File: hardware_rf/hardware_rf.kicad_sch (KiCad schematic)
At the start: 5 parts, among them IC1 CC1125RHBR, Y1 Crystal_GND24

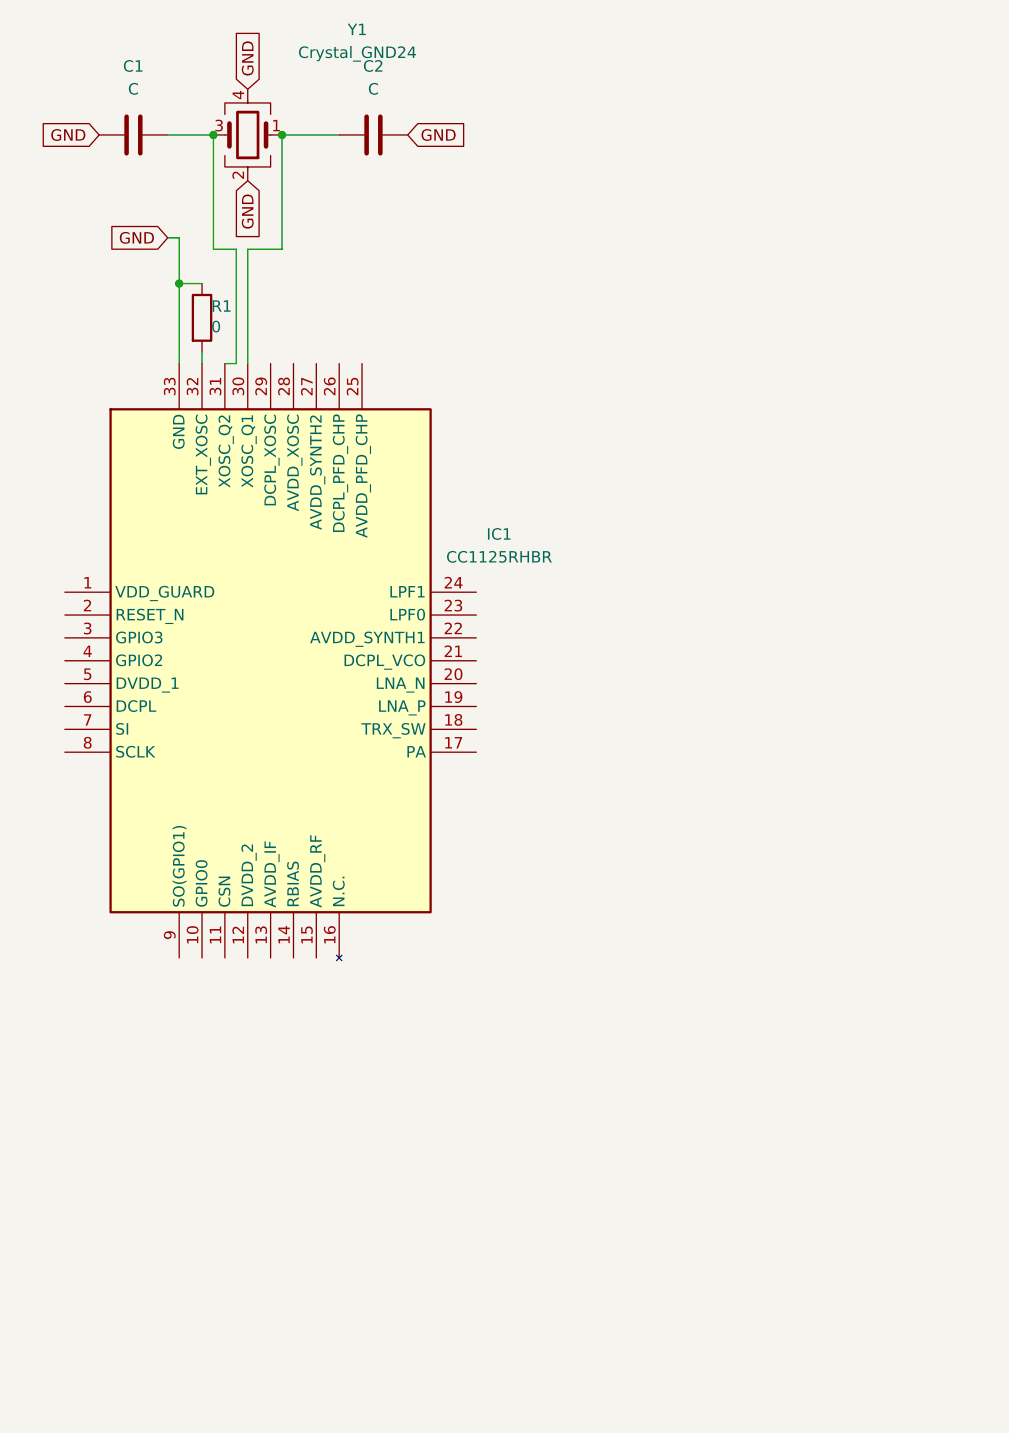
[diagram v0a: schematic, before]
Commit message: schematic work
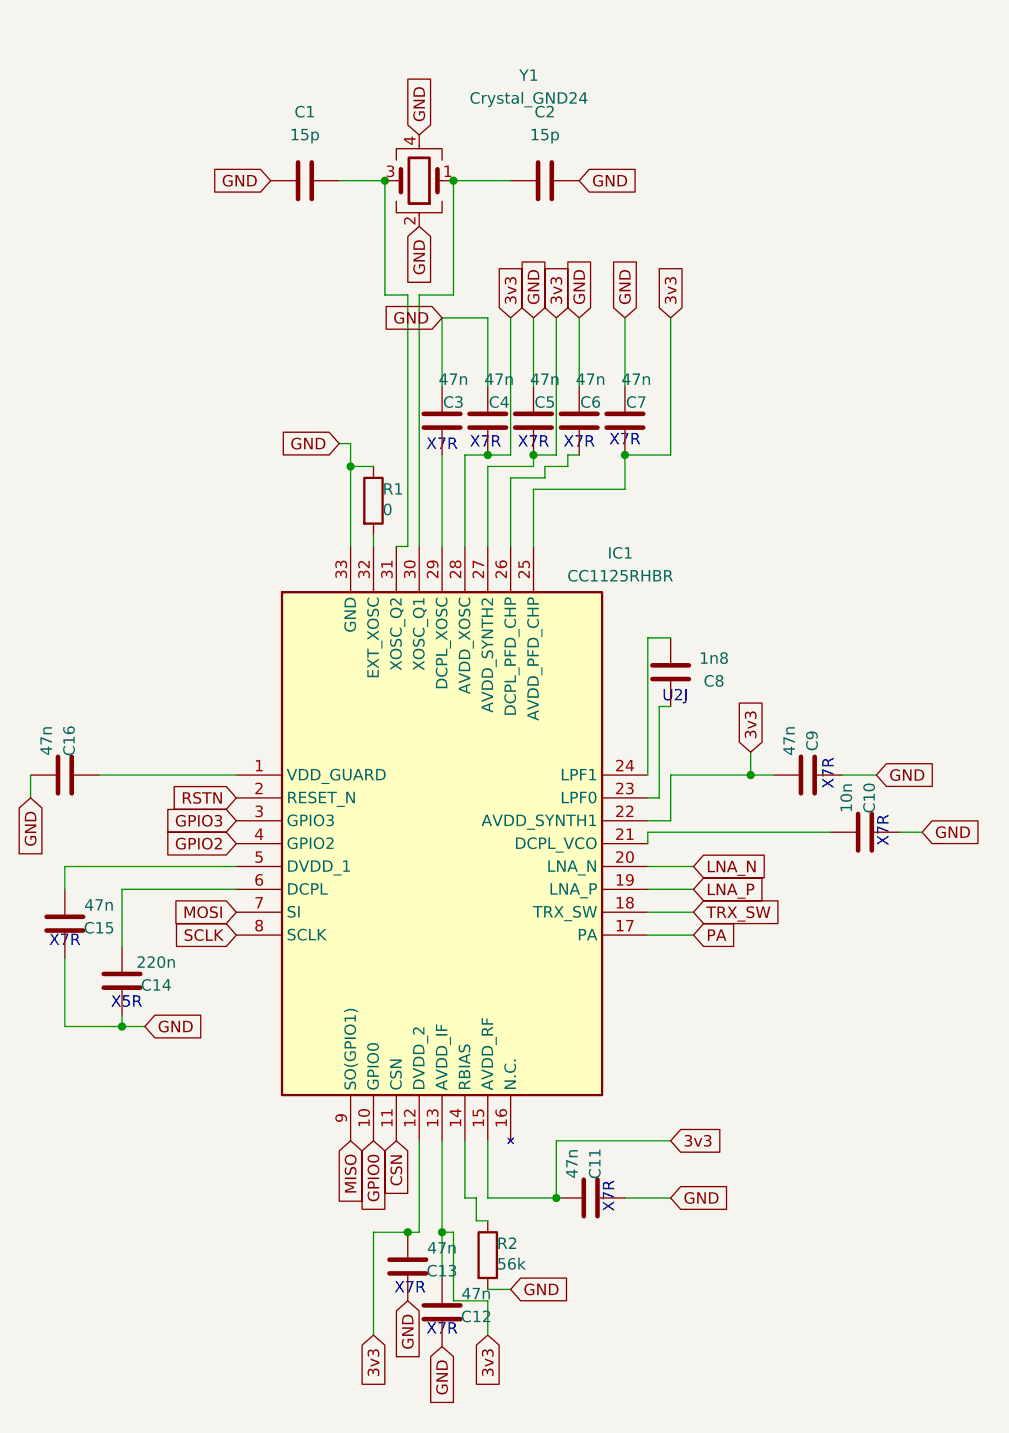
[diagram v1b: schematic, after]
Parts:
- added C10: 10n, symbol Device:C
- added C11, C12, C13, C15, C16, C3, C4, C5, C6, C7, C9: 47n, symbol Device:C
- added C14: 220n, symbol Device:C
- added C8: 1n8, symbol Device:C
- added R2: 56k, symbol Device:R
- C1, C2: value C -> 15p
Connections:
- net GND: now also C10.2, C11.2, C12.2, C13.2, C14.2, C15.2, C16.1, C3.1, C4.1, C5.1, C6.1, C7.1, C9.2, R2.2
- net at IC1.1 (VDD_GUARD): now also C16.2
- net GPIO0: now reaches IC1.10 (GPIO0)
- net CSN: now reaches IC1.11 (CSN)
- net 3v3: now reaches IC1.12 (DVDD_2)
- net 3v3: now also IC1.13 (AVDD_IF), IC1.15 (AVDD_RF), IC1.22 (AVDD_SYNTH1), IC1.25 (AVDD_PFD_CHP), IC1.27 (AVDD_SYNTH2), IC1.28 (AVDD_XOSC), C11.1, C12.1, C13.1, C4.2, C5.2, C7.2, C9.1
- net at IC1.14 (RBIAS): now also R2.1
- net PA: now reaches IC1.17 (PA)
- net TRX_SW: now reaches IC1.18 (TRX_SW)
- net LNA_P: now reaches IC1.19 (LNA_P)
- net RSTN: now reaches IC1.2 (RESET_N)
- net LNA_N: now reaches IC1.20 (LNA_N)
- net at IC1.21 (DCPL_VCO): now also C10.1
- net at IC1.23 (LPF0): now also C8.2
- net at IC1.24 (LPF1): now also C8.1
- net at IC1.26 (DCPL_PFD_CHP): now also C6.2
- net at IC1.29 (DCPL_XOSC): now also C3.2
- net GPIO3: now reaches IC1.3 (GPIO3)
- net GPIO2: now reaches IC1.4 (GPIO2)
- net at IC1.5 (DVDD_1): now also C15.1
- net at IC1.6 (DCPL): now also C14.1
- net MOSI: now reaches IC1.7 (SI)
- net SCLK: now reaches IC1.8 (SCLK)
- net MISO: now reaches IC1.9 (SO(GPIO1))
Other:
- note added: "U2J"
- note added: "X5R"
- note added: "X7R"
- moved on the sheet: C1, C2, IC1, R1, Y1

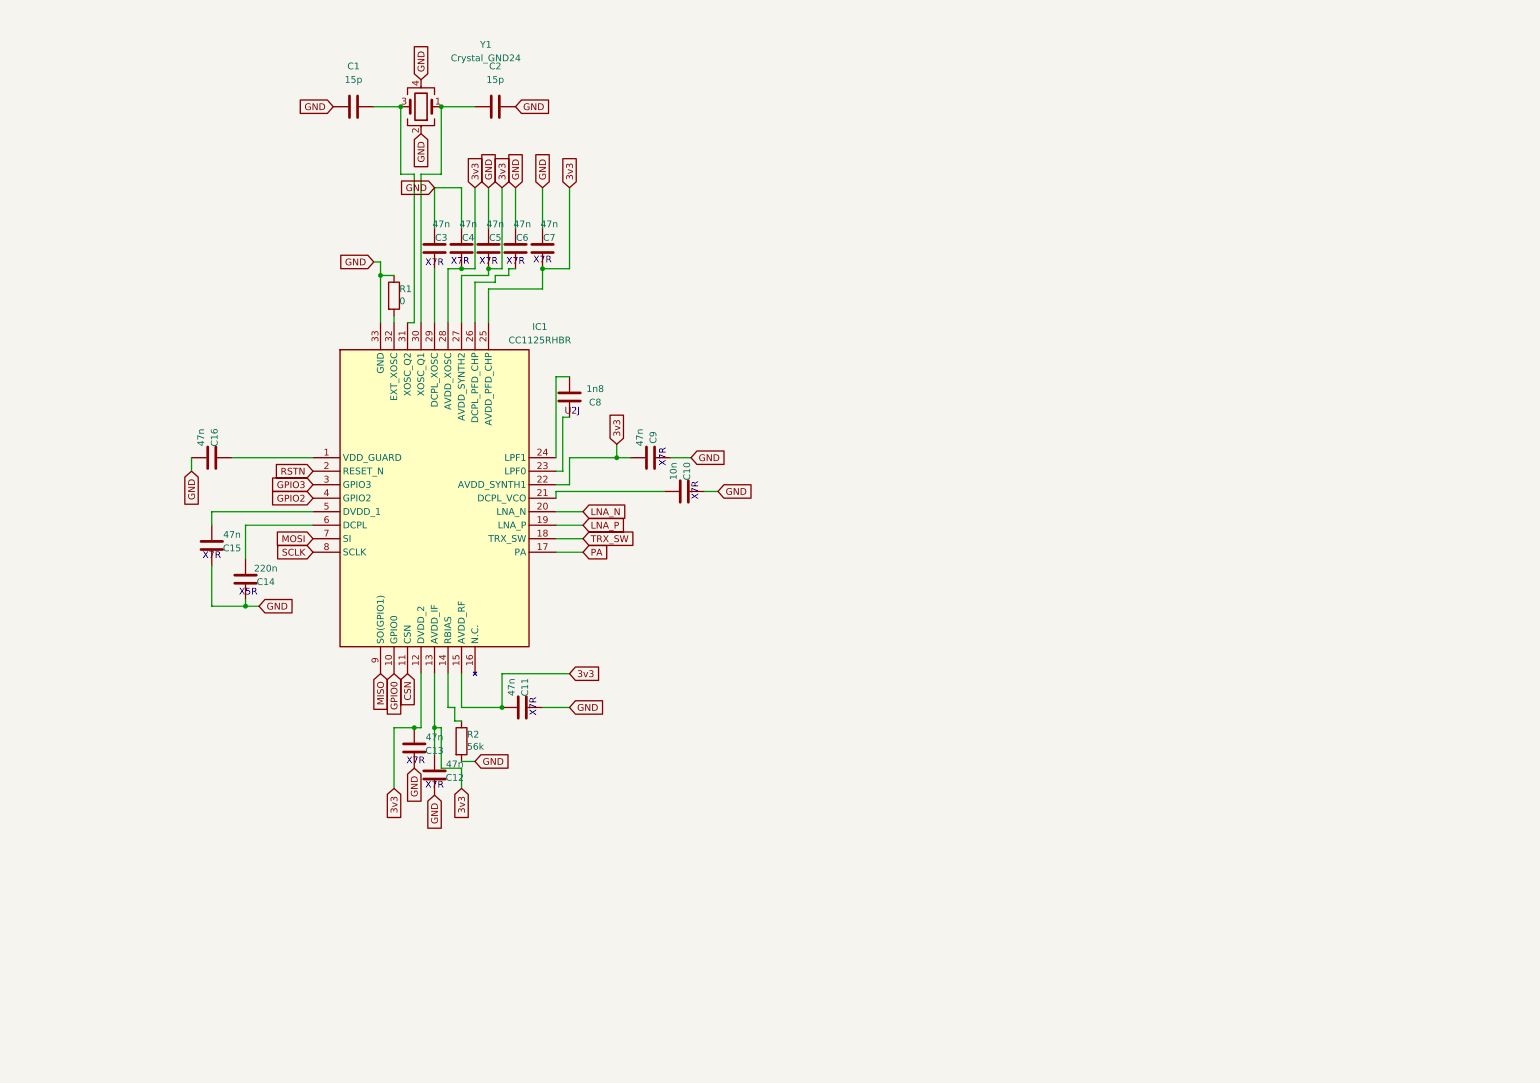
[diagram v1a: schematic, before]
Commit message: pcb
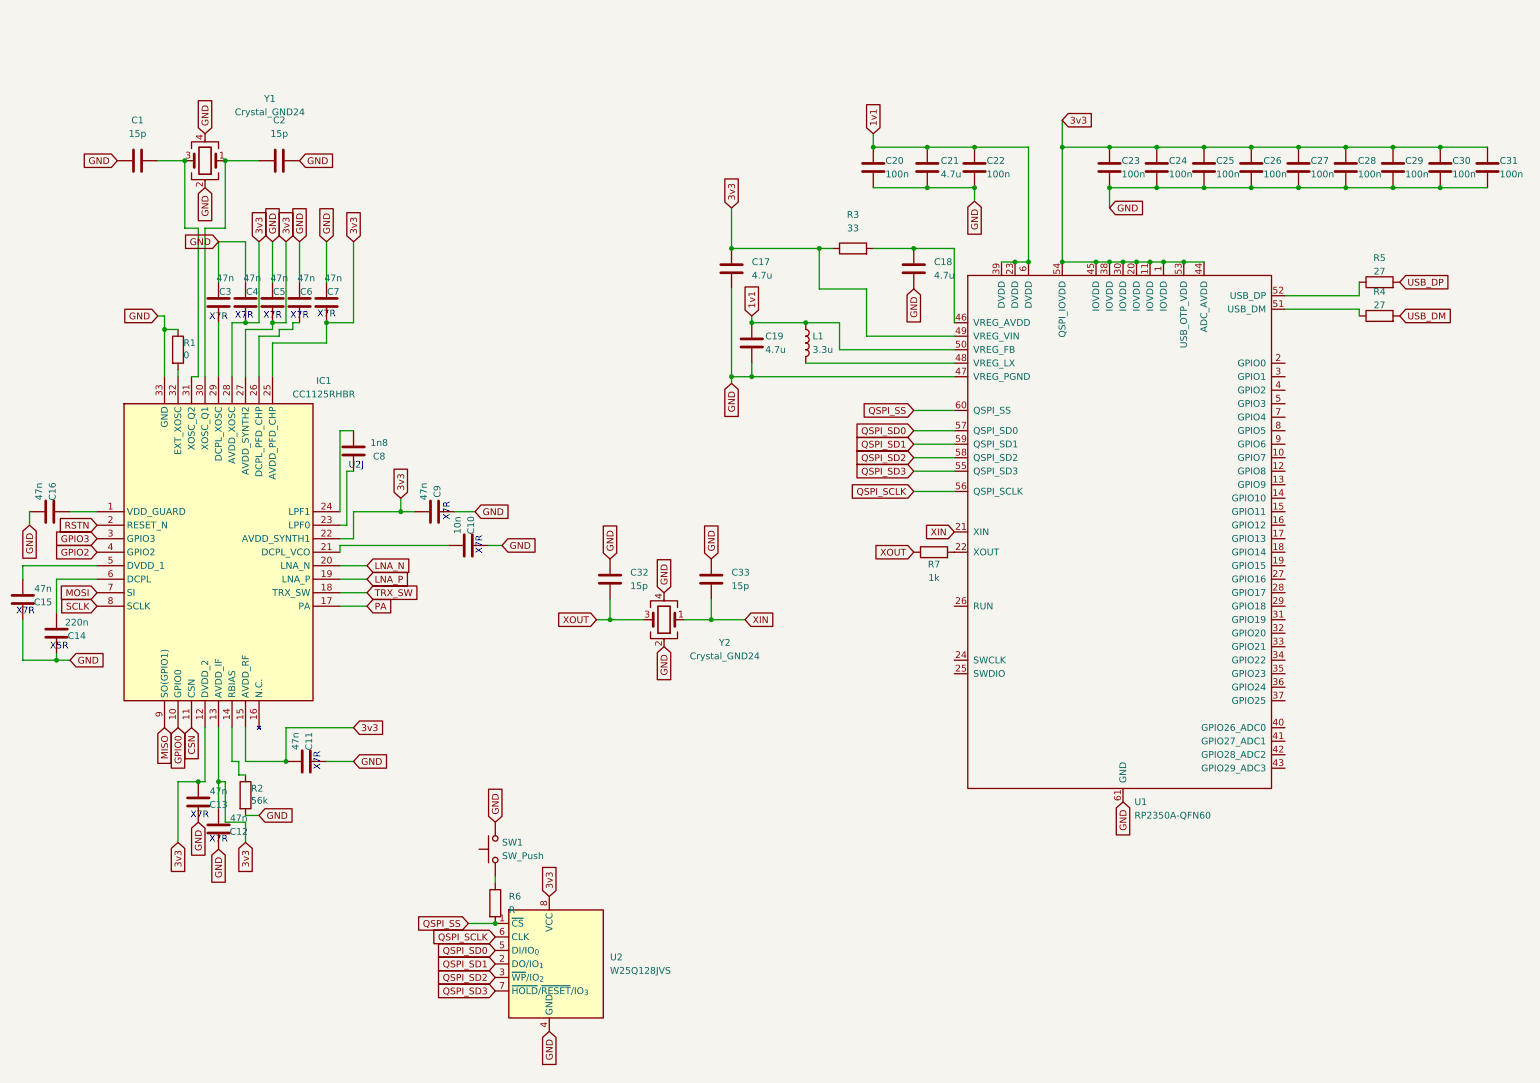
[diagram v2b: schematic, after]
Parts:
- added C17, C18, C19, C21: 4.7u, symbol Device:C
- added C20, C22, C23, C24, C25, C26, C27, C28, C29, C30, C31: 100n, symbol Device:C
- added C32, C33: 15p, symbol Device:C
- added L1: 3.3u, symbol Device:L
- added R3: 33, symbol Device:R
- added R4, R5: 27, symbol Device:R
- added R6: R, symbol Device:R
- added R7: 1k, symbol Device:R
- added SW1: SW_Push, symbol Switch:SW_Push
- added U1: RP2350A-QFN60, mainfoot:RP2350A_QFN-60_EP_7.75x7.75_Pitch0.4mm, symbol mainlib:RP2350A-QFN60
- added U2: W25Q128JVS, Package_SO:SOIC-8_5.3x5.3mm_P1.27mm, symbol Memory_Flash:W25Q128JVS
- added Y2: Crystal_GND24, symbol Device:Crystal_GND24
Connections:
- net 3v3: now also C17.1, C23.1, C24.1, C25.1, C26.1, C27.1, C28.1, C29.1, C30.1, C31.1, R3.1, U1.1 (IOVDD), U1.11 (IOVDD), U1.20 (IOVDD), U1.30 (IOVDD), U1.38 (IOVDD), U1.44 (ADC_AVDD), U1.45 (IOVDD), U1.49 (VREG_VIN), U1.53 (USB_OTP_VDD), U1.54 (QSPI_IOVDD), U2.8 (VCC)
- net GND: now also C17.2, C18.2, C19.2, C20.2, C21.2, C22.2, C23.2, C24.2, C25.2, C26.2, C27.2, C28.2, C29.2, C30.2, C31.2, C32.1, C33.1, SW1.2, U1.47 (VREG_PGND), U1.61 (GND), U2.4 (GND), Y2.2, Y2.4
- new net: R7.2, U1.22 (XOUT)
- new net: C18.1, R3.2, U1.46 (VREG_AVDD)
- new net: L1.2, U1.48 (VREG_LX)
- new net: R4.1, U1.51 (USB_DM)
- new net: R5.1, U1.52 (USB_DP)
- new net: R6.1, SW1.1
- new net 1v1: C19.1, C20.1, C21.1, C22.1, L1.1, U1.23 (DVDD), U1.39 (DVDD), U1.50 (VREG_FB), U1.6 (DVDD)
- new net QSPI_SCLK: U1.56 (QSPI_SCLK), U2.6 (CLK)
- new net QSPI_SD0: U1.57 (QSPI_SD0), U2.5 (DI/IO_{0})
- new net QSPI_SD1: U1.59 (QSPI_SD1), U2.2 (DO/IO_{1})
- new net QSPI_SD2: U1.58 (QSPI_SD2), U2.3 (~{WP}/IO_{2})
- new net QSPI_SD3: U1.55 (QSPI_SD3), U2.7 (~{HOLD}/~{RESET}/IO_{3})
- new net QSPI_SS: R6.2, U1.60 (QSPI_SS), U2.1 (~{CS})
- new net USB_DM: R4.2
- new net USB_DP: R5.2
- new net XIN: C33.2, U1.21 (XIN), Y2.1
- new net XOUT: C32.2, R7.1, Y2.3
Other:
- title: (none) -> RF Board For VikramSAT
- moved on the sheet: C1, C10, C11, C12, C13, C14, C15, C16, C2, C3, C4, C5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
